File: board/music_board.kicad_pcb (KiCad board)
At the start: 2 copper layers, 100 x 70 mm, 10 parts, among them J1 Conn_01x07, SW1 RotaryEncoder_Switch_MP, SW2 RotaryEncoder_Switch_MP, U1 Waveshare ESP32-S3-ZERO

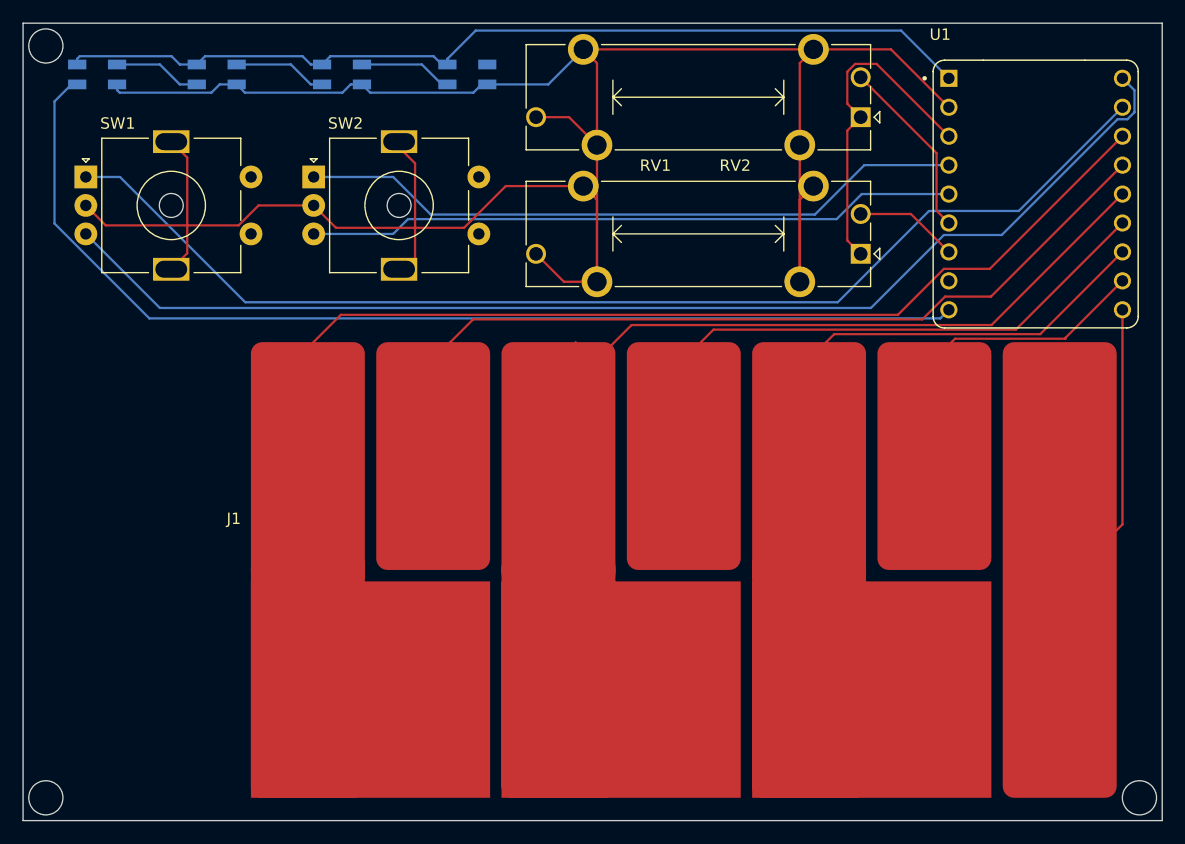
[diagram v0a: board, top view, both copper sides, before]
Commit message: Add files via upload
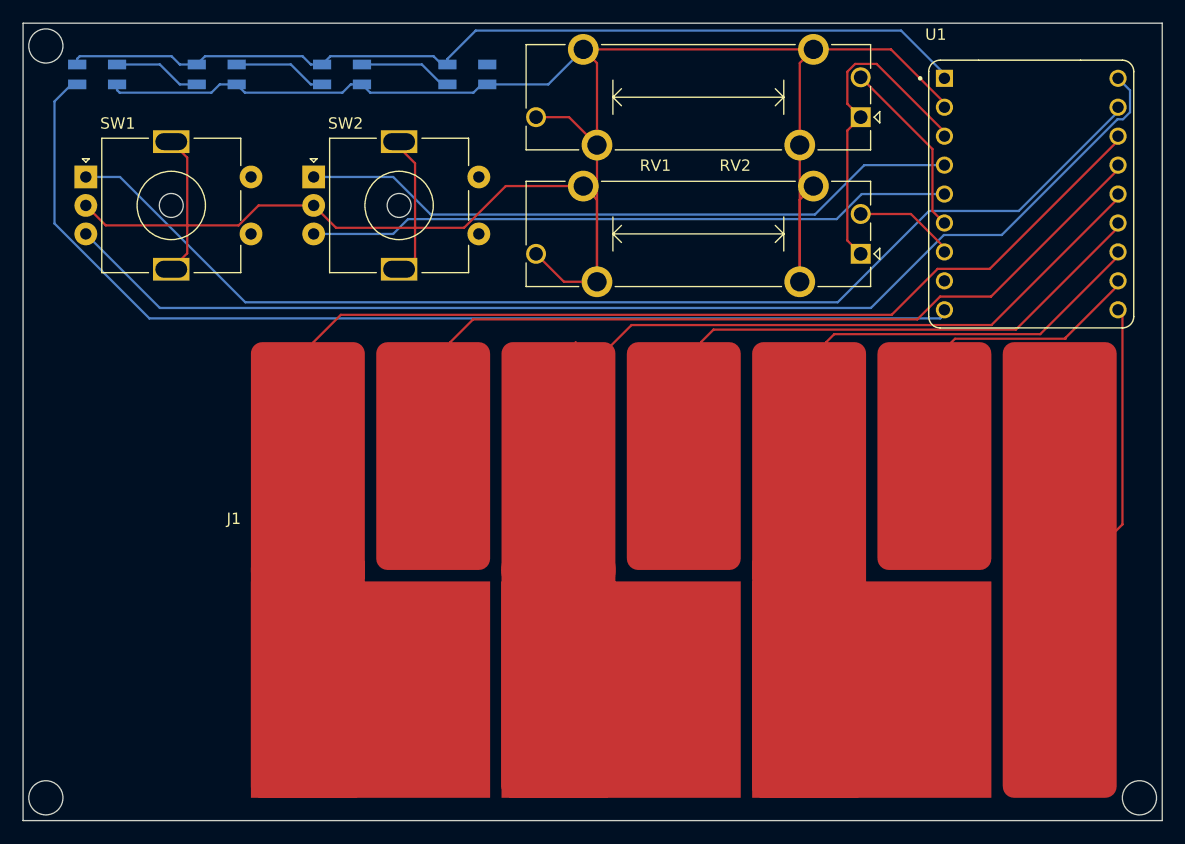
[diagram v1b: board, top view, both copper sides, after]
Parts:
- moved U1 0.39 mm to (202.5, 91.0)
